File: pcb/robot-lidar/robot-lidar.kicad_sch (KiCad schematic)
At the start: 48 parts, among them J2 YLIDAR X4, J3 Jack-DC, J5 Conn_01x02, J5 Conn_02x03_Odd_Even, J6 Conn_01x02, J7 Conn_01x02, J7 Conn_ARM_SWD_TagConnect_TC2030, J8 Conn_01x02, SW1 SW_SPST, U1 STM32F429VETx, U2 LM317-3.3_SOT-223, U2 MPU-6050, U4 MX1508, U5 MX1508, Y1 Crystal

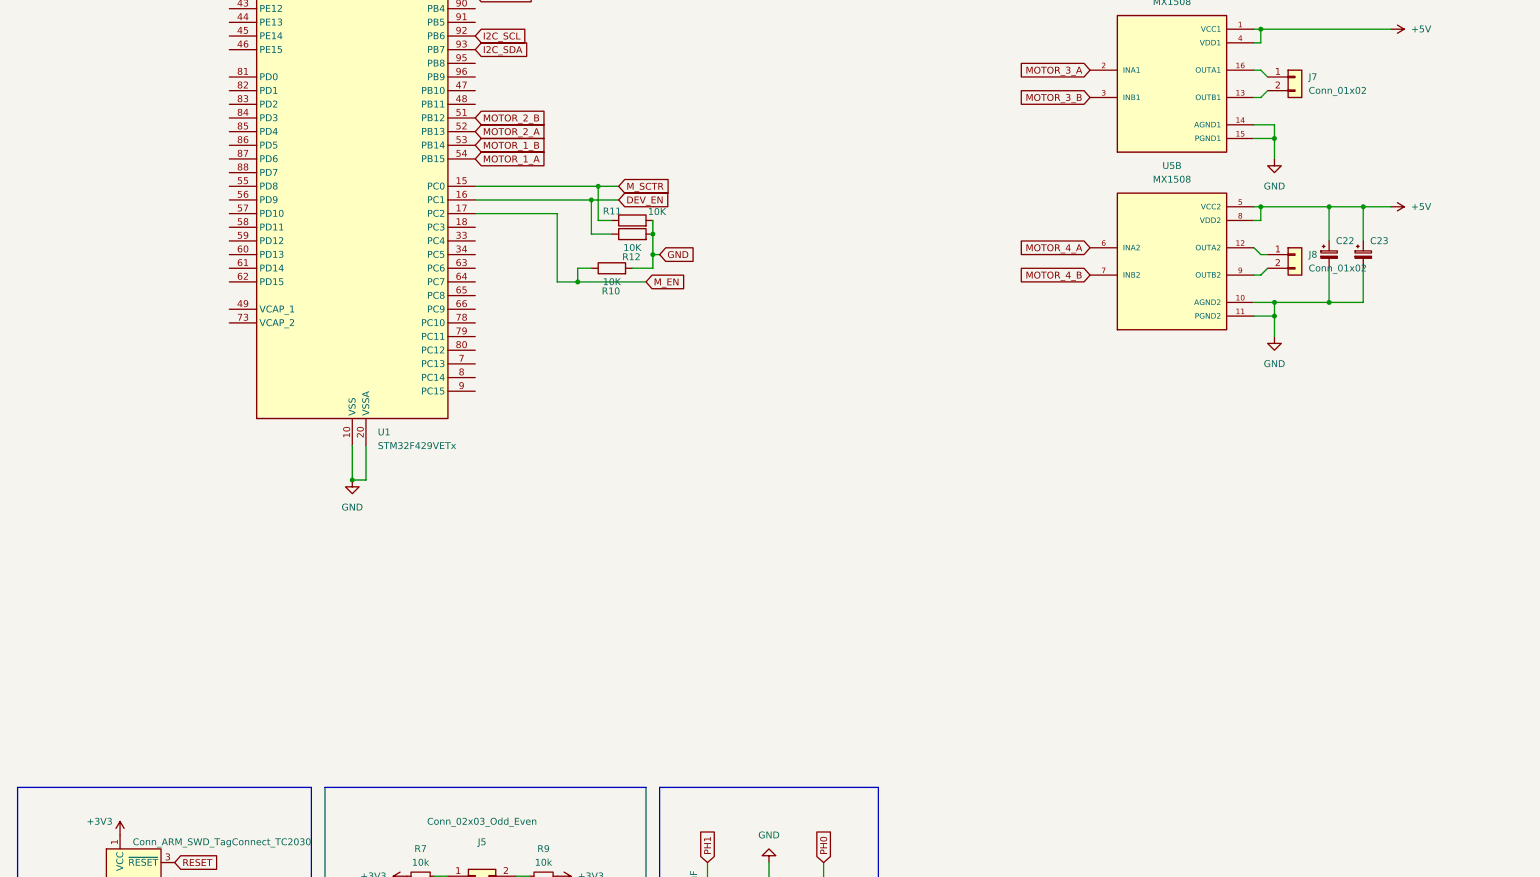
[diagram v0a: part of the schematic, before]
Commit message: add linkit
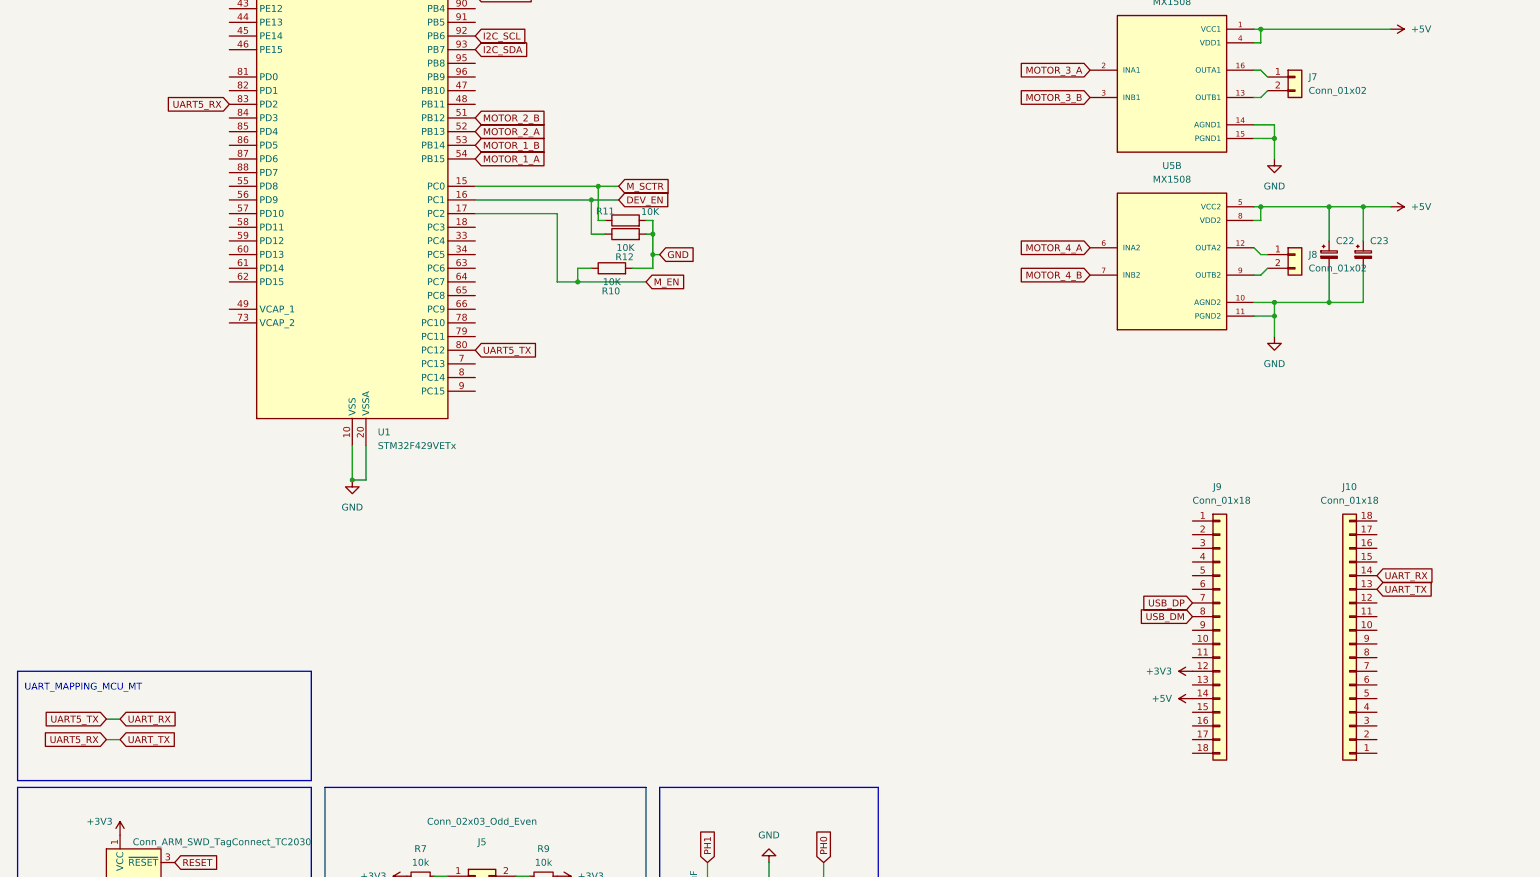
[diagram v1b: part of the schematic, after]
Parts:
- added J10, J9: Conn_01x18, symbol Connector_Generic:Conn_01x18
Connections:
- net +3V3: now also J9.12 (Pin_12)
- net +5V: now also J9.14 (Pin_14)
- net UART5_TX: now reaches U1.80 (PC12)
- net UART5_TX: now also J10.14 (Pin_14)
- net UART5_RX: now reaches U1.83 (PD2)
- net UART5_RX: now also J10.13 (Pin_13)
- new net USB_DM: J9.8 (Pin_8)
- new net USB_DP: J9.7 (Pin_7)
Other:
- note added: "UART_MAPPING_MCU_MT"
- moved on the sheet: R11, R12
